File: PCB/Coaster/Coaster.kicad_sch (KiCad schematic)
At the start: 138 parts, among them J1 USB-C, J2 Shelly, J3 Join, P1 TestPoint, P10 TestPoint, P11 TestPoint, P12 TestPoint, P2 TestPoint, P3 TestPoint, P4 TestPoint, P5 TestPoint, P6 TestPoint, P7 TestPoint, P8 TestPoint, P9 TestPoint, T1 TestPoint, T10 TestPoint, T11 TestPoint, T12 TestPoint, T2 TestPoint, T3 TestPoint, T4 TestPoint, T5 TestPoint, T6 TestPoint, T7 TestPoint, T8 TestPoint, T9 TestPoint, U1 ESP32-PICO-MINI-02, U2 LMR16006XDDCR, U3 QR

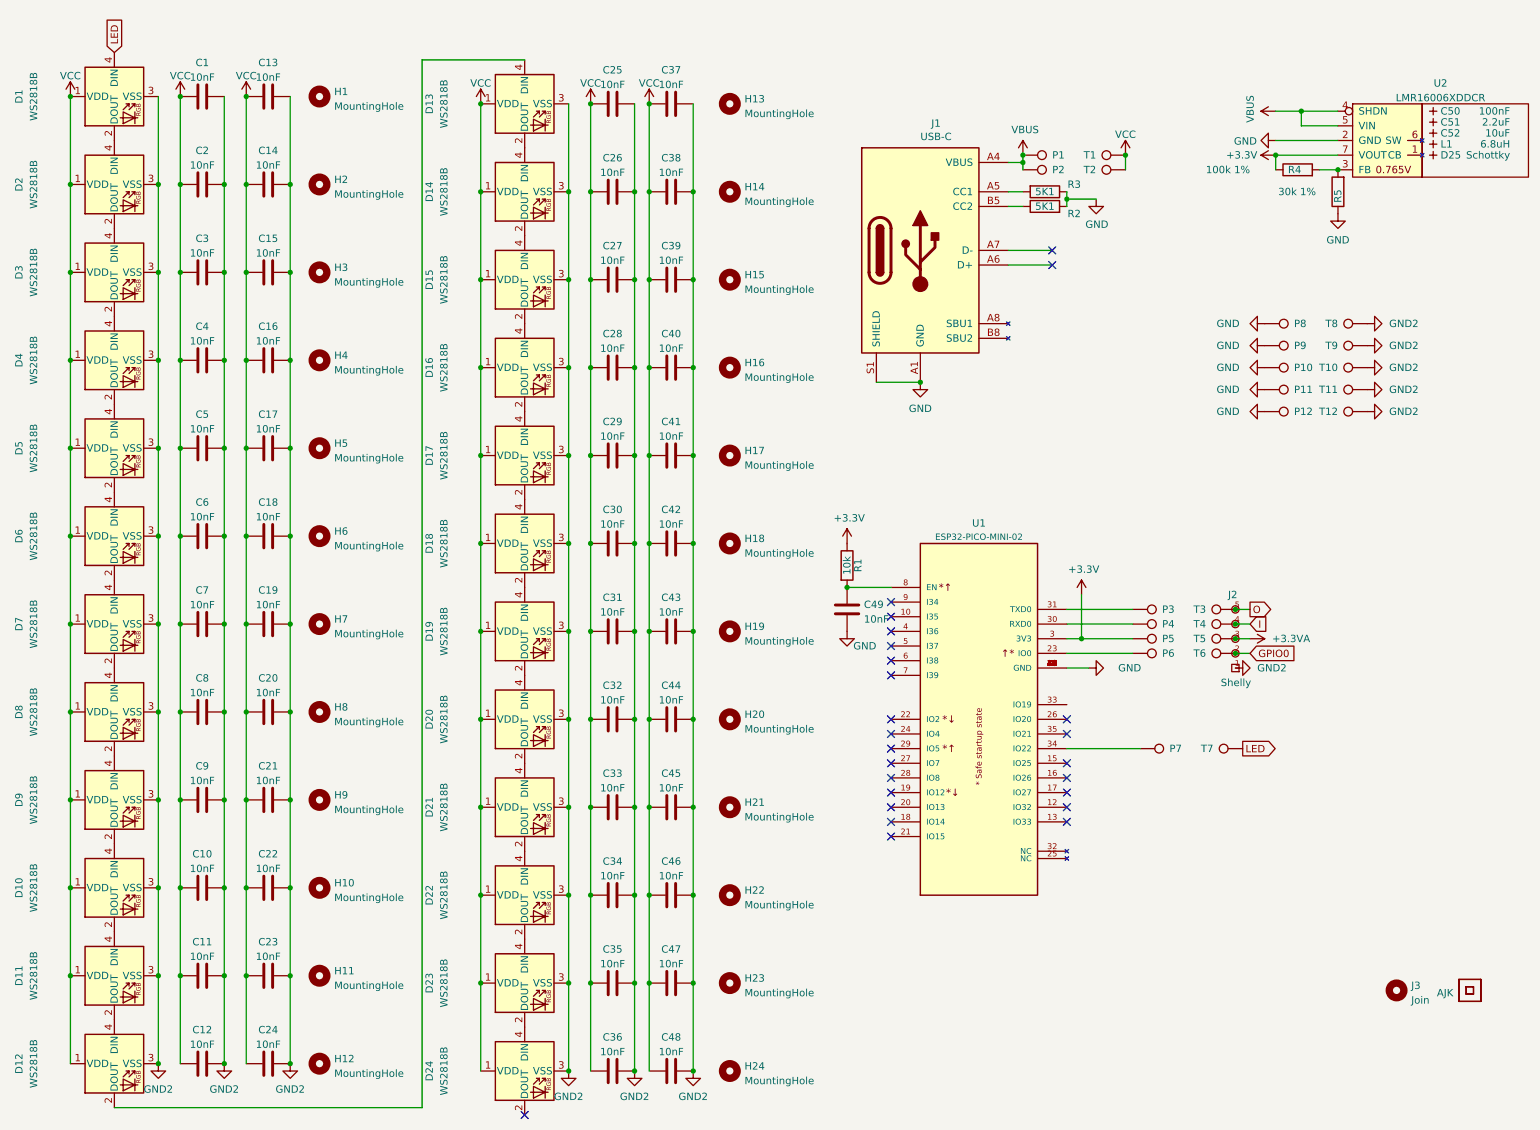
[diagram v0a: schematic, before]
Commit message: Arrrg
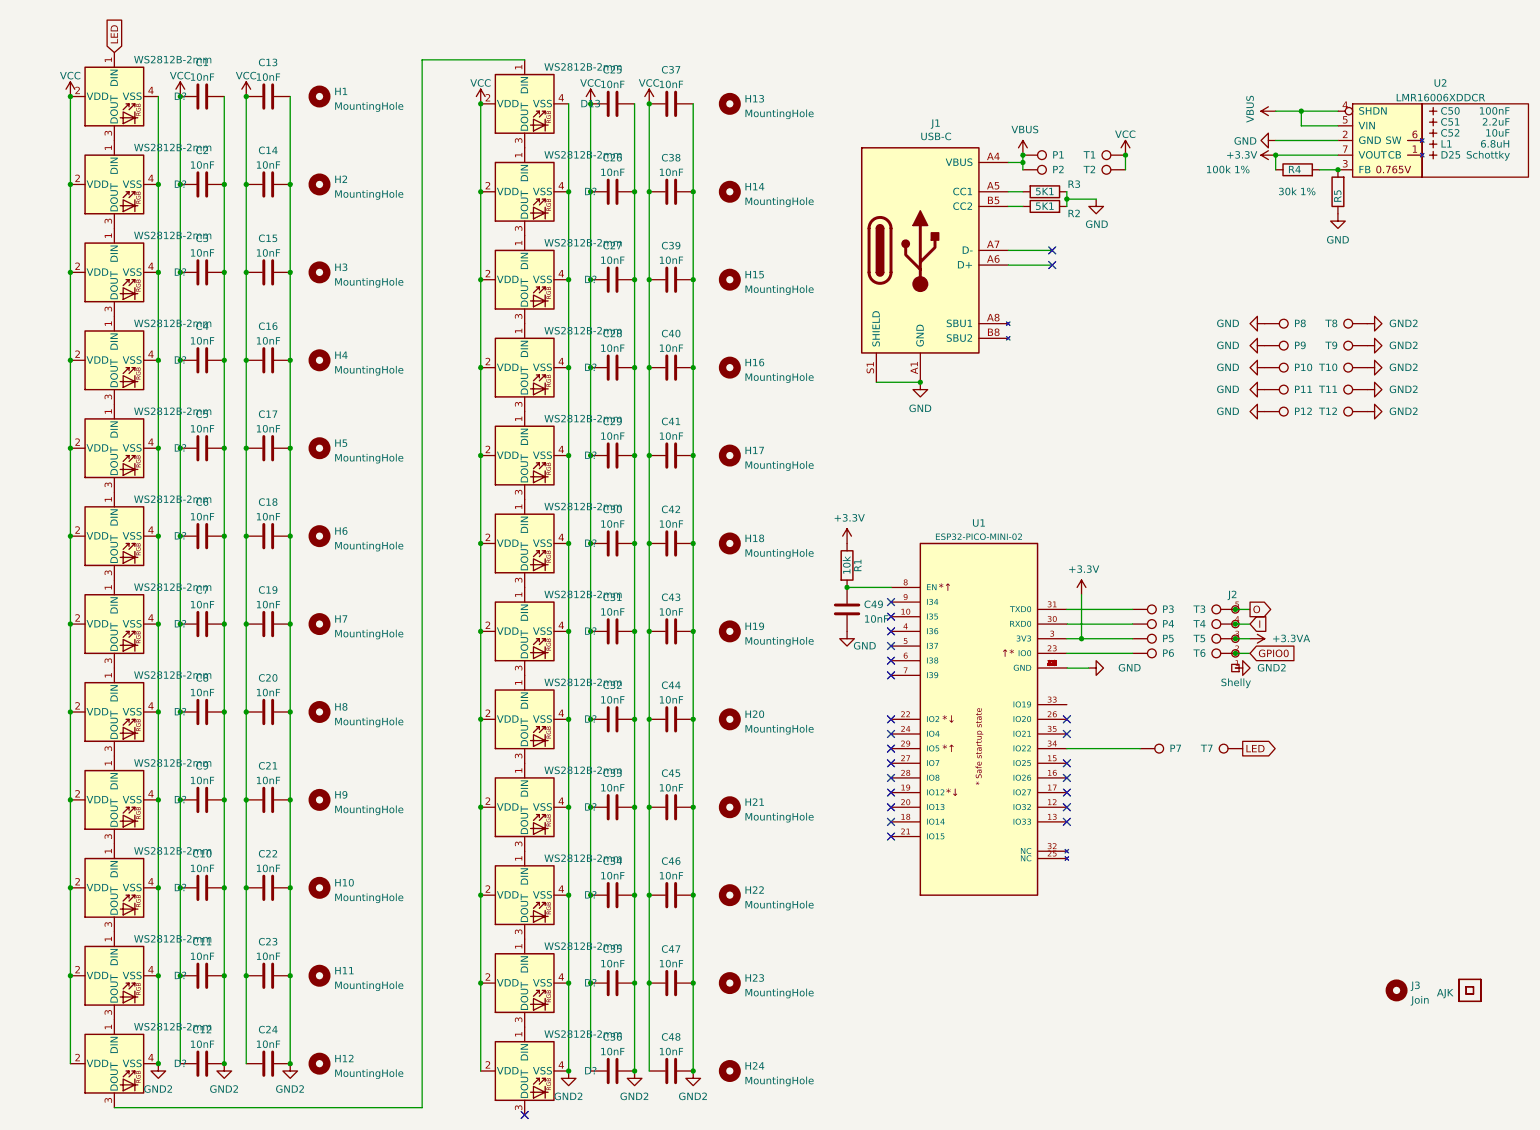
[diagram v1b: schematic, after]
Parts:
- removed D1, D10, D11, D12, D13, D14, D15, D16, D17, D18, D19, D2, D20, D21, D22, D23, D24, D3, D4, D5, D6, D7, D8, D9: WS2818B, RevK:SMD2020, symbol LED:WS2812B
- added D13, D? (x23): WS2812B-2mm, RevK:SMD2020, symbol RevK:WS2812B-2mm
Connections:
- net GND2: now also D13.4 (VSS), D?.4 (VSS), D?.4 (VSS), D?.4 (VSS), D?.4 (VSS), D?.4 (VSS), D?.4 (VSS), D?.4 (VSS), D?.4 (VSS), D?.4 (VSS), D?.4 (VSS), D?.4 (VSS), D?.4 (VSS), D?.4 (VSS), D?.4 (VSS), D?.4 (VSS), D?.4 (VSS), D?.4 (VSS), D?.4 (VSS), D?.4 (VSS), D?.4 (VSS), D?.4 (VSS), D?.4 (VSS), D?.4 (VSS)
- net LED: now also D?.1 (DIN)
- net VCC: now also D13.2 (VDD), D?.2 (VDD), D?.2 (VDD), D?.2 (VDD), D?.2 (VDD), D?.2 (VDD), D?.2 (VDD), D?.2 (VDD), D?.2 (VDD), D?.2 (VDD), D?.2 (VDD), D?.2 (VDD), D?.2 (VDD), D?.2 (VDD), D?.2 (VDD), D?.2 (VDD), D?.2 (VDD), D?.2 (VDD), D?.2 (VDD), D?.2 (VDD), D?.2 (VDD), D?.2 (VDD), D?.2 (VDD), D?.2 (VDD)
- new net: D?.1 (DIN), D?.3 (DOUT) (x21)
- new net: D13.3 (DOUT), D?.1 (DIN)
- new net: D13.1 (DIN), D?.3 (DOUT)
